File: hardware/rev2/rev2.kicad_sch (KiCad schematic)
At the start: 49 parts, among them J1 USB_C_Receptacle_USB2.0_16P, J2 uFL, J3 uFL, J4 Antenna RF and GNSS Data, J5 Antenna GND, J7 uFL, U1 EClamp2522P

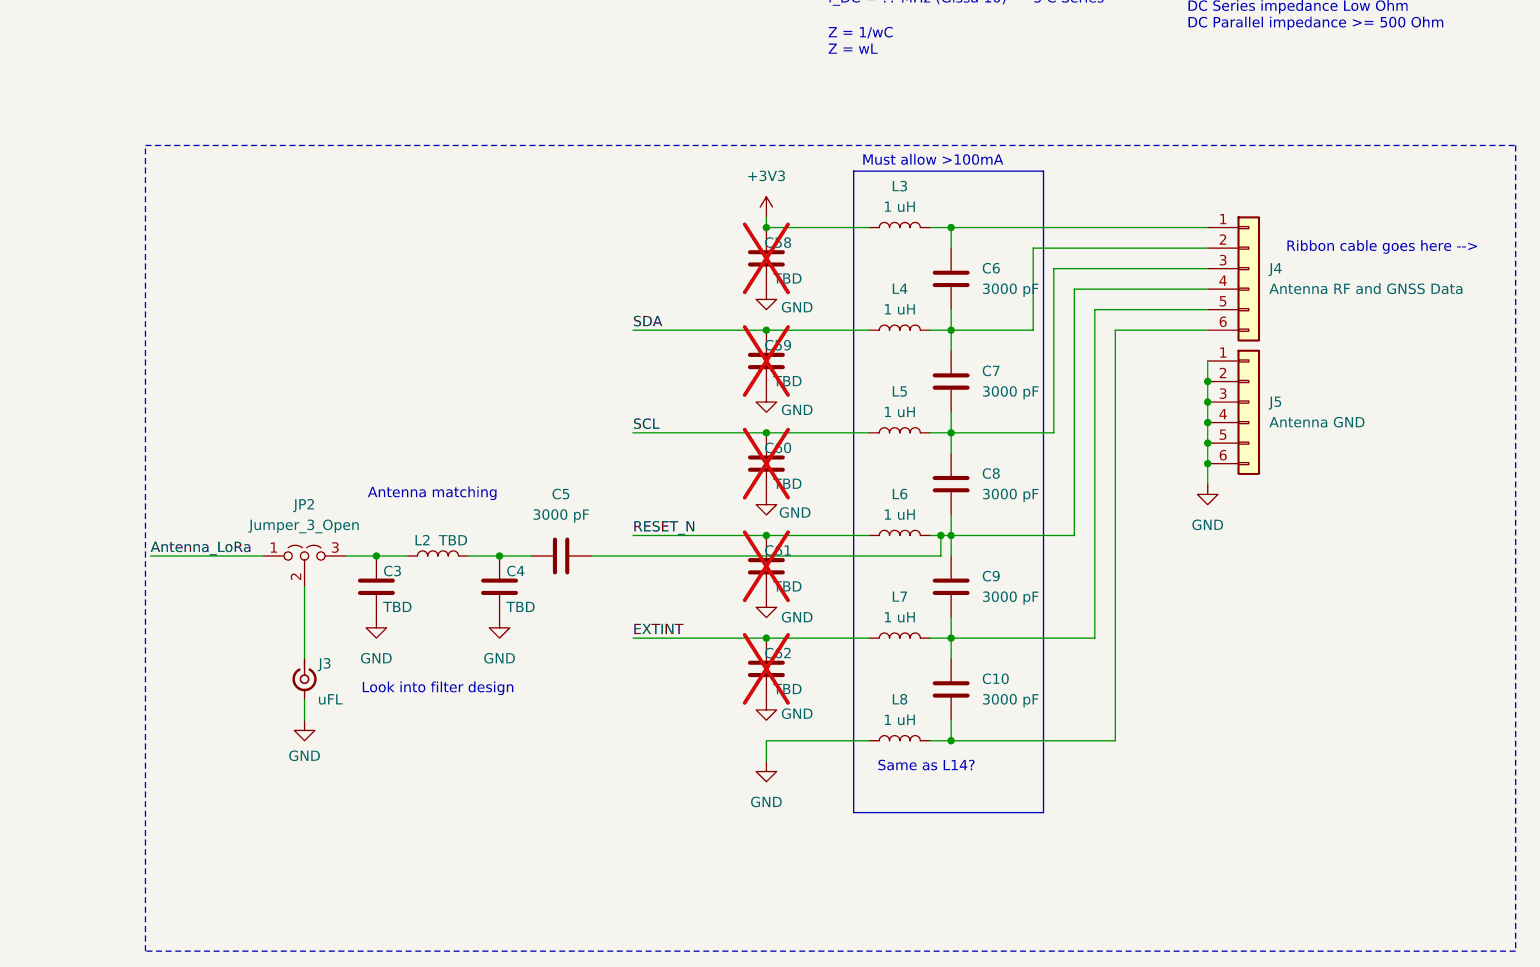
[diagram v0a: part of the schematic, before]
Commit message: final edit, send to production
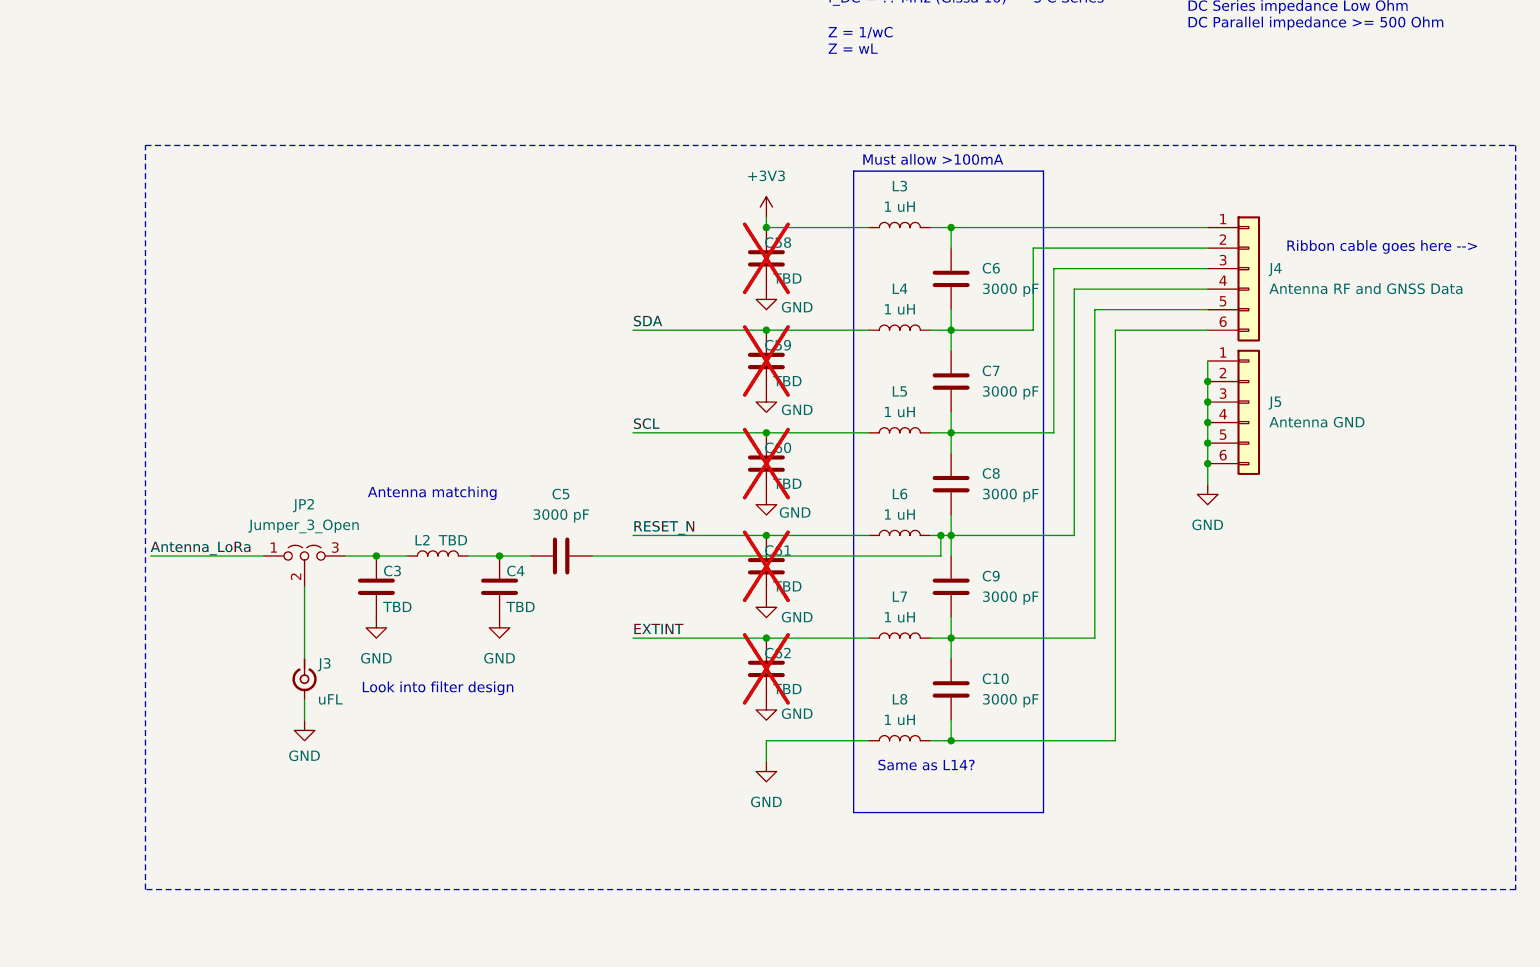
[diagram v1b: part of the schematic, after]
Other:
- company: MMCX11 -> Group 10
- title: (none) -> LoRa Based Cat Tracker
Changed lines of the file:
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@@
 	(paper "A3")
 	(title_block
-		(company "MMCX11")
+		(title "LoRa Based Cat Tracker")
+		(date "2026-04-22")
+		(rev "2.0.0")
+		(company "Group 10")
+		(comment 1 "MMCX11")
 	)
 	(rectangle
@@
 	(rectangle
 		(start 233.045 158.75)
-		(end 402.59 258.445)
+		(end 402.59 250.825)
 		(stroke
 			(width 0)
